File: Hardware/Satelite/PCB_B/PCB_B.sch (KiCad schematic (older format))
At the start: 11 parts, among them IC1 MCP1642B-50I_MS, J1 Conector_PCB_B-C, J2 Conector_PCB_A-B, U1 MIC5323-3.3YD5_TR

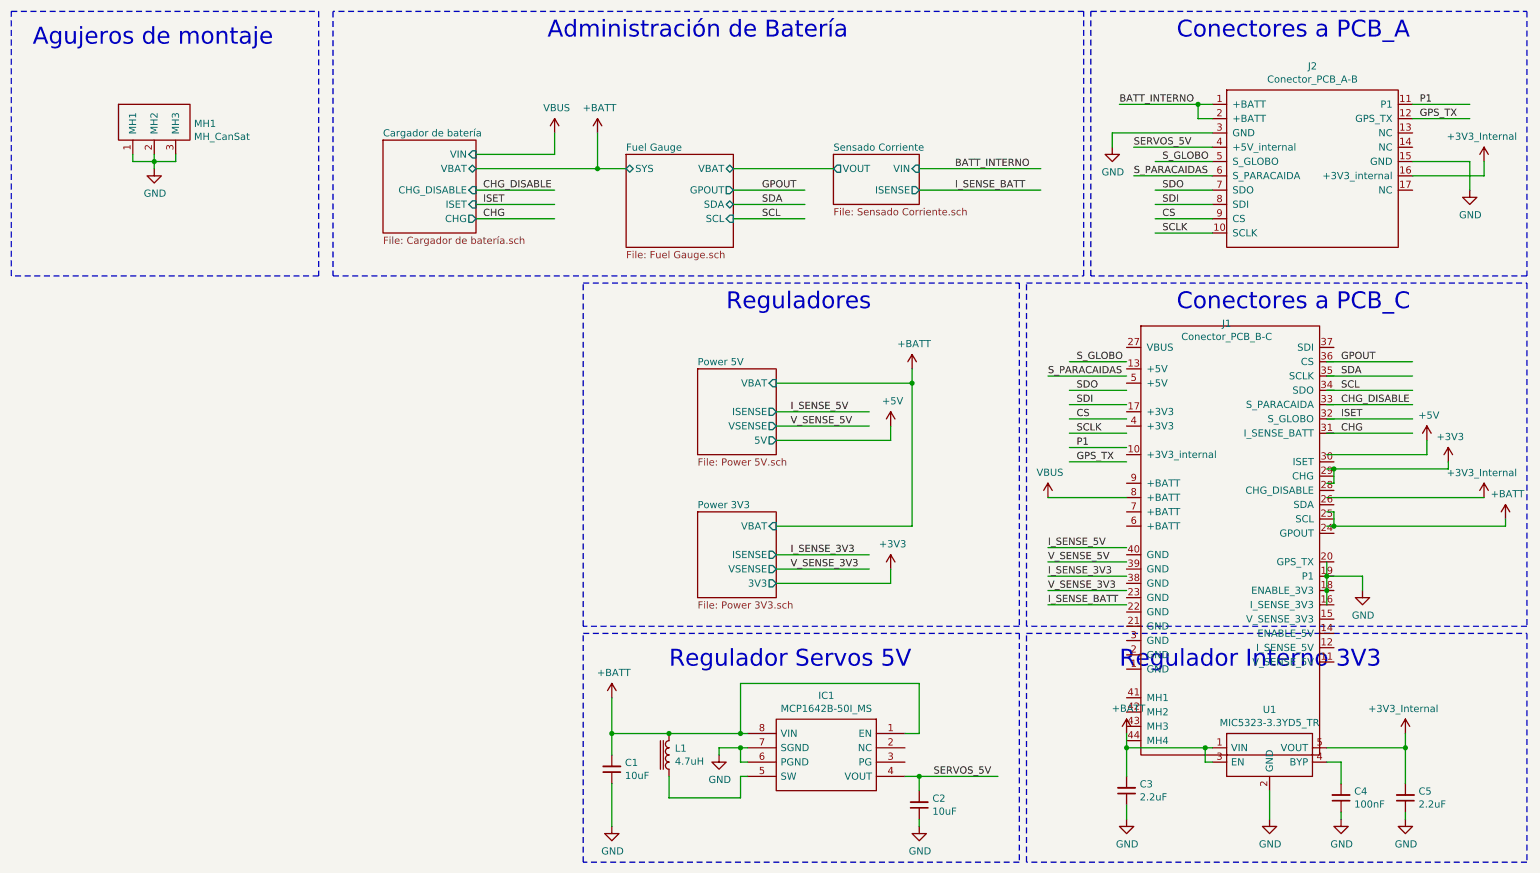
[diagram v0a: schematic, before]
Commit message: Nuevo conector B-C
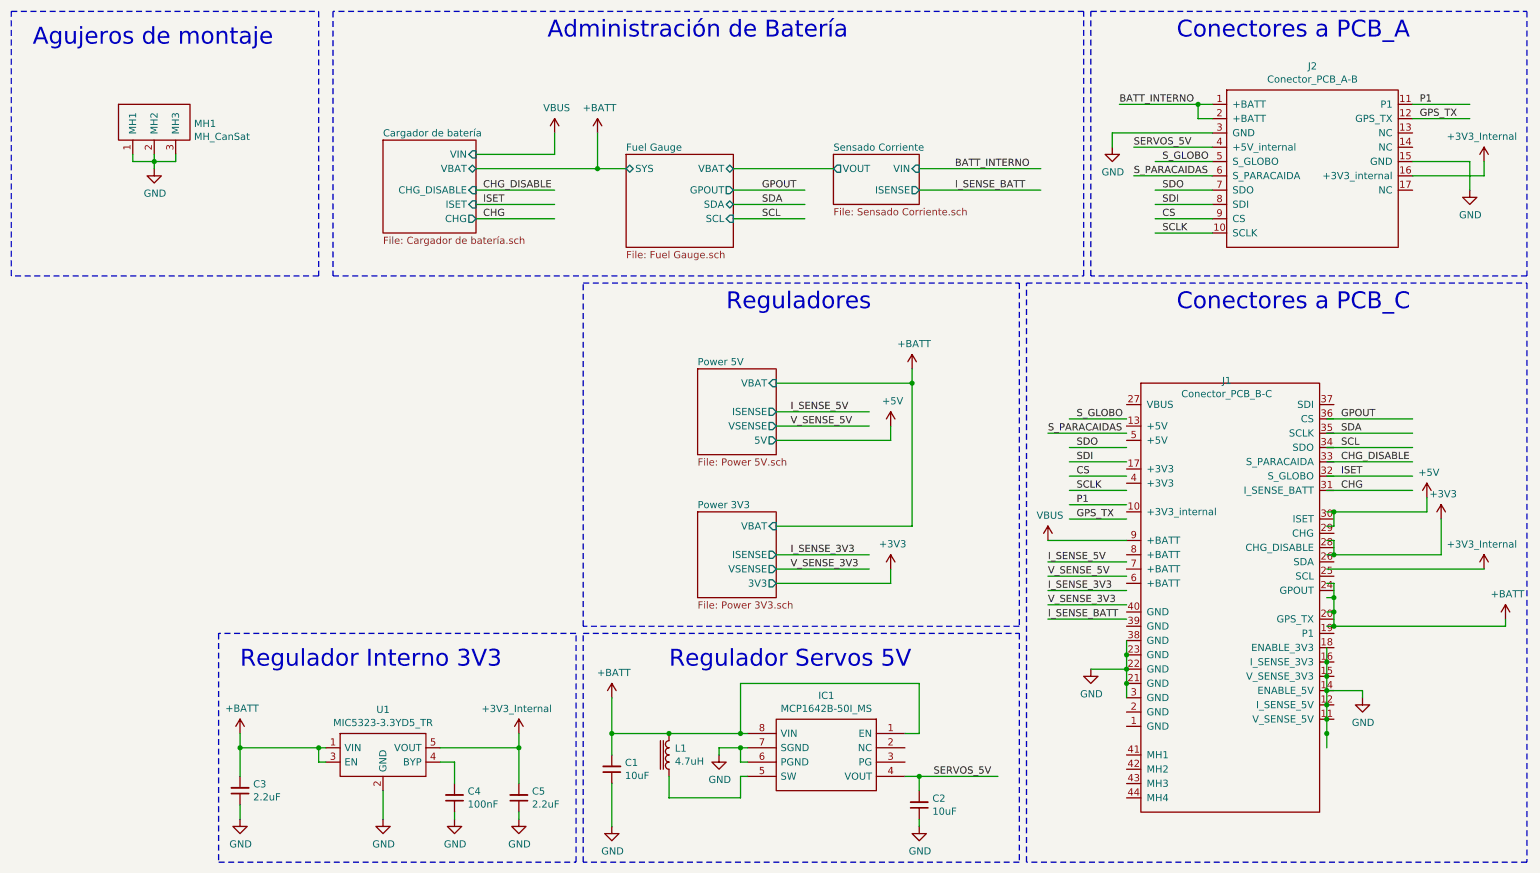
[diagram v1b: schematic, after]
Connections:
- wire segments 127 -> 143
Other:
- moved on the sheet: C3, C4, C5, J1, U1
